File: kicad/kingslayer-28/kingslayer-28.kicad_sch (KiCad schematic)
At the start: 96 parts, among them IC1 STM32F303CCT7, IC2 IS31FL3731-QFLS2-TR, K1 KEYSW, K10 KEYSW, K11 KEYSW, K12 KEYSW, K13 KEYSW, K14 KEYSW, K15 KEYSW, K16 KEYSW, K17 KEYSW, K18 KEYSW, K19 KEYSW, K2 KEYSW, K20 KEYSW, K21 KEYSW, K22 KEYSW, K23 KEYSW, K24 KEYSW, K25 KEYSW, K26 KEYSW, K27 KEYSW, K28 KEYSW, K3 KEYSW, K4 KEYSW, K5 KEYSW, K6 KEYSW, K7 KEYSW, K8 KEYSW, K9 KEYSW, SW1 SW_PUSH, X1 XTAL_GND

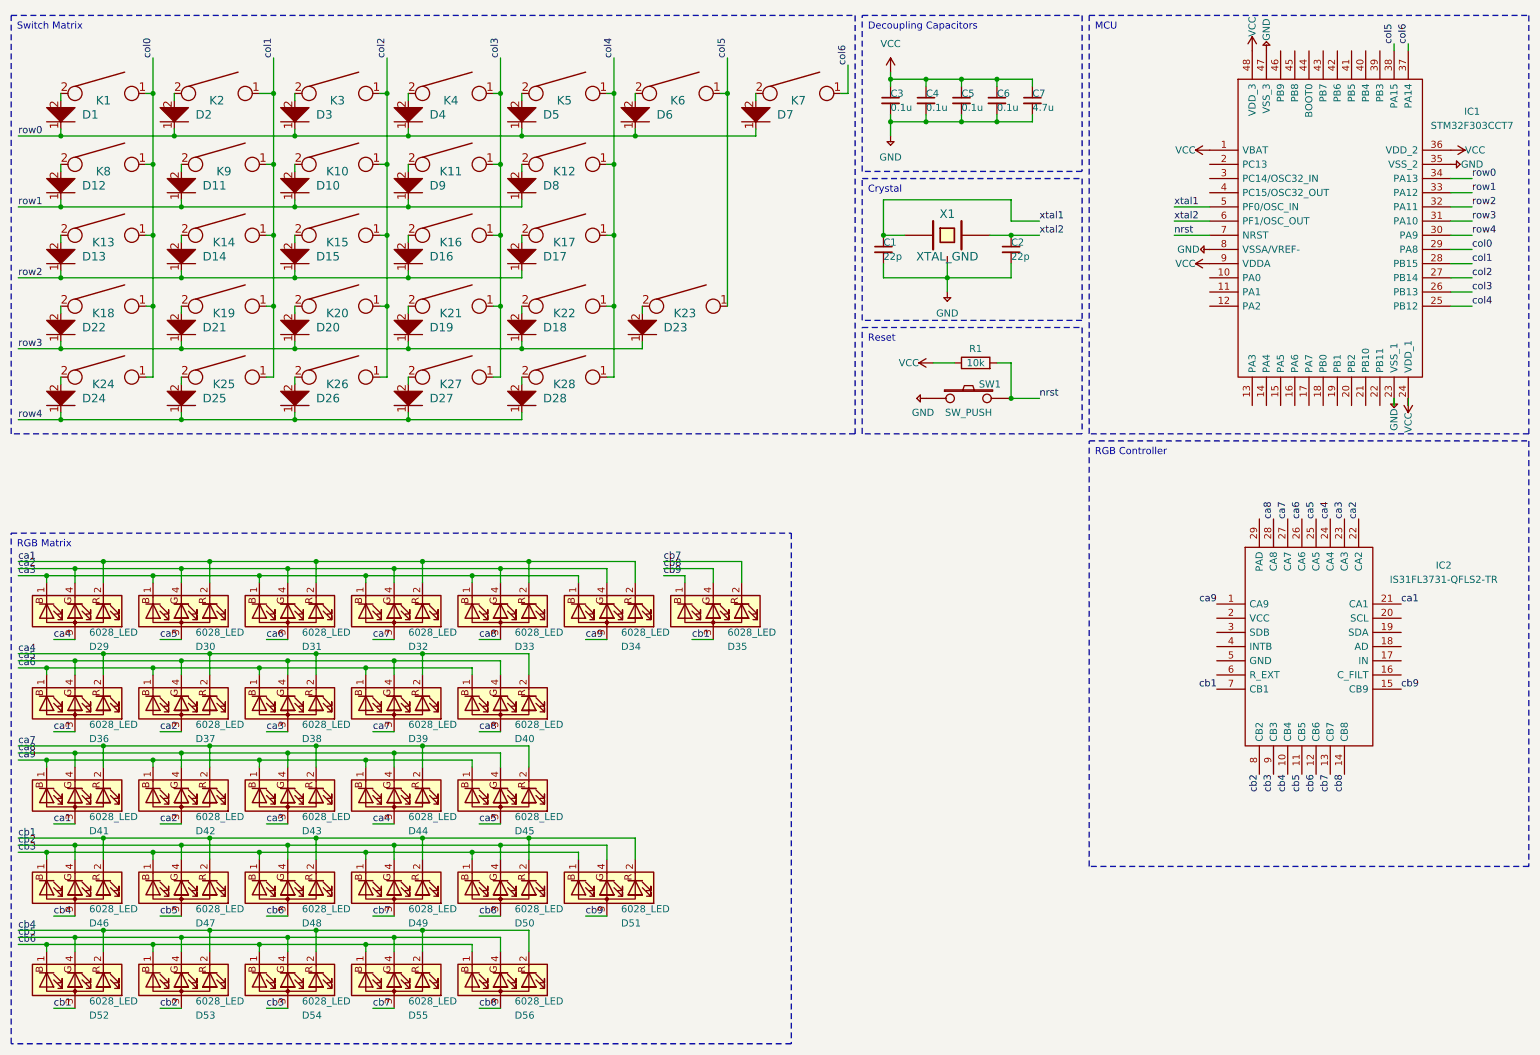
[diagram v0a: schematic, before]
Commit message: USB C
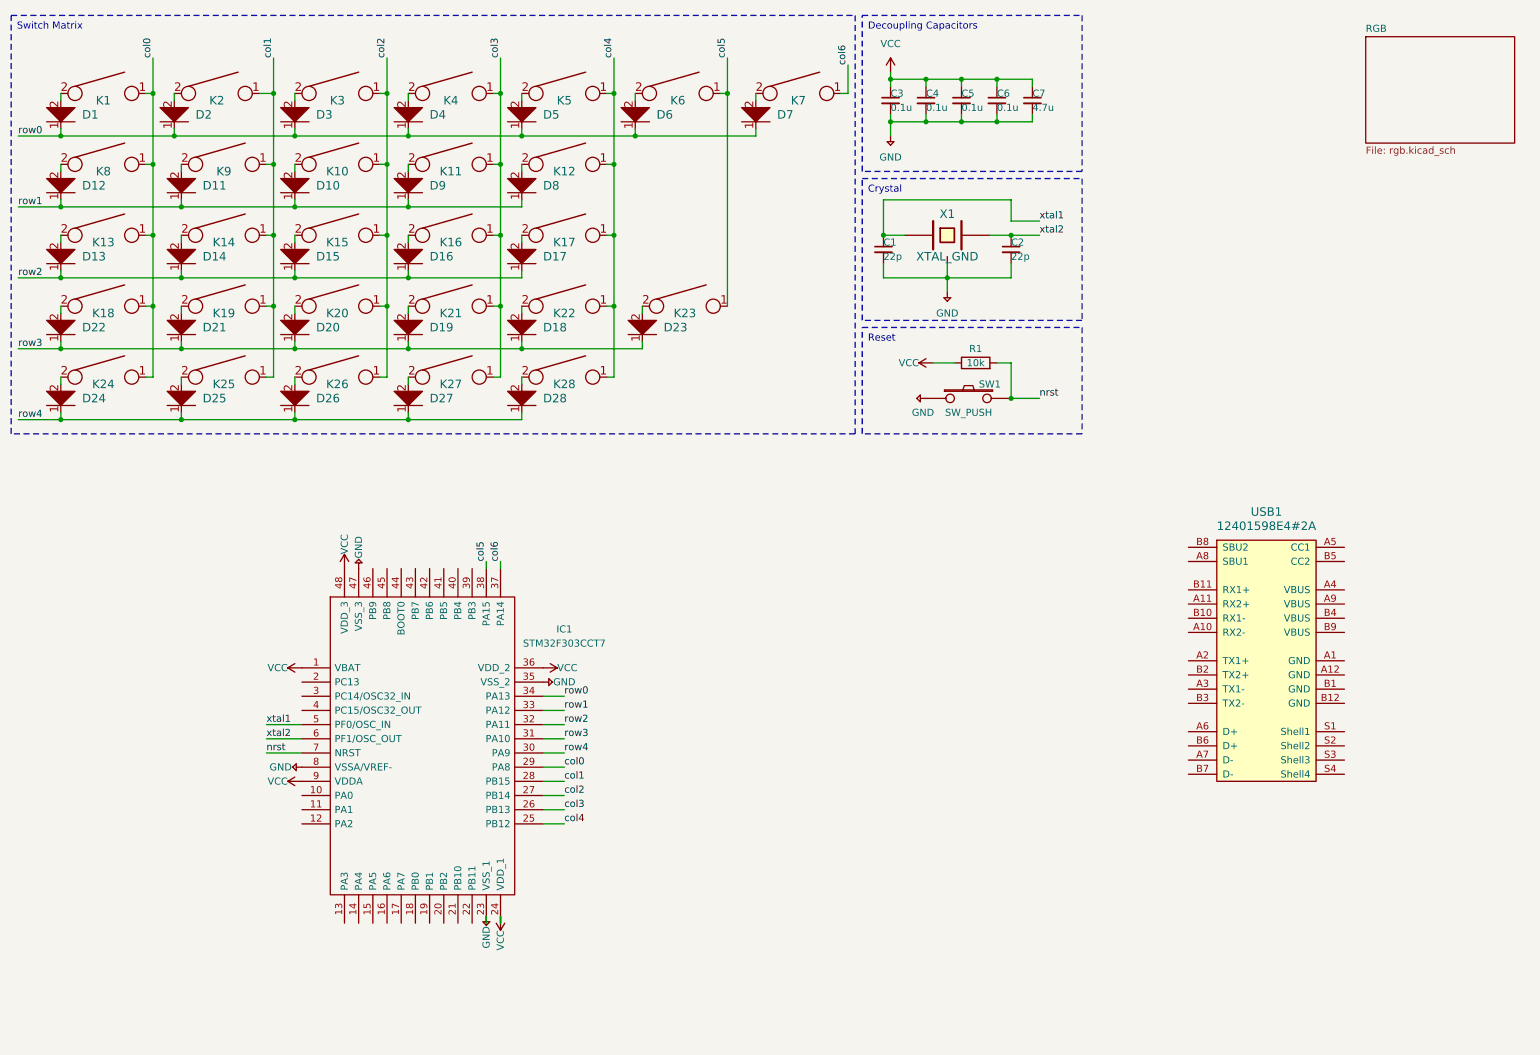
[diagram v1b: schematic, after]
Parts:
- removed D29, D30, D31, D32, D33, D34, D35, D36, D37, D38, D39, D40, D41, D42, D43, D44, D45, D46, D47, D48, D49, D50, D51, D52, D53, D54, D55, D56: 6028_LED, symbol Device:LED_BRAG
- removed IC2: IS31FL3731-QFLS2-TR, QFN40P400X400X80-29N, symbol IS31FL3731-QFLS2-TR:IS31FL3731-QFLS2-TR
- added USB1: 12401598E4#2A, symbol Type-C:12401598E4#2A
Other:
- added sheet RGB (rgb.kicad_sch)
- moved on the sheet: IC1
